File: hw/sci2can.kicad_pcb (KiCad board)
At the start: 2 copper layers, 31.1 x 32 mm, 34 parts, among them IC1 MC9S08DZ60xLC, J1 BDM, J2 Screw Terminal, Q1 4MHz, Q2 MGSF1N03L*, U1 uA7805, U2 PCA82C251

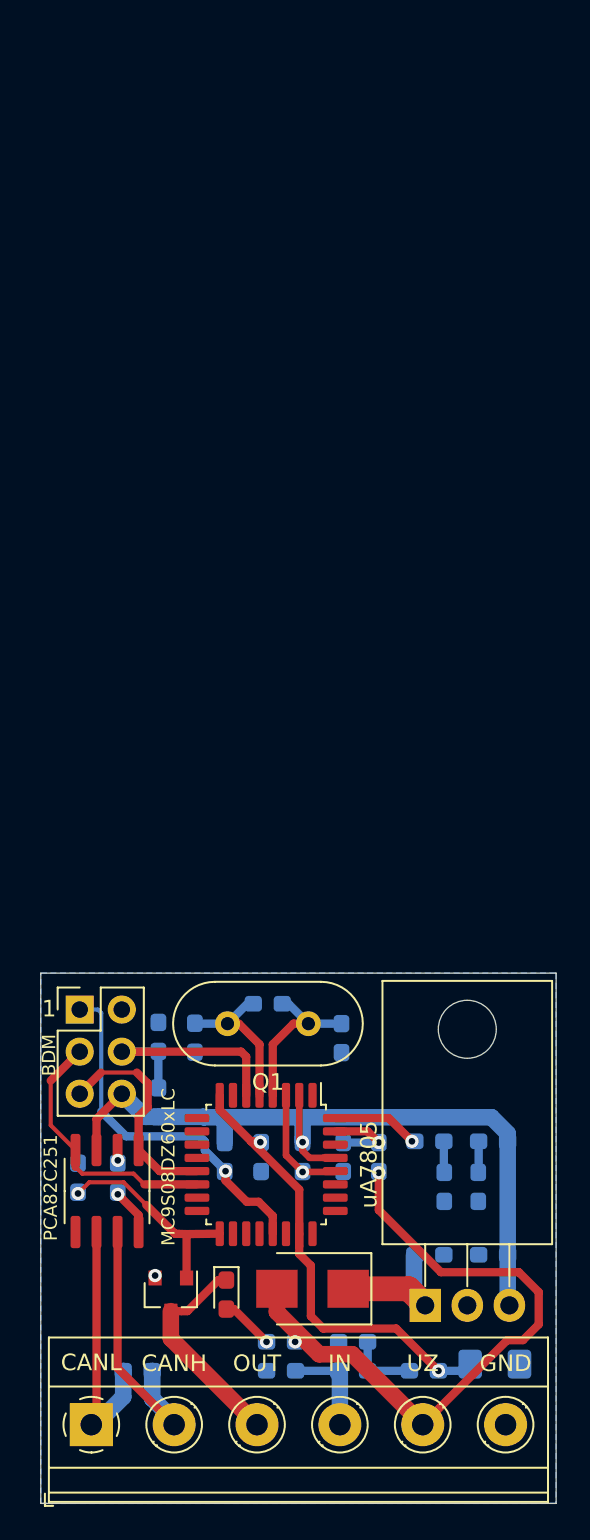
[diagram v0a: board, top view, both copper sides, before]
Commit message: hw 1v02
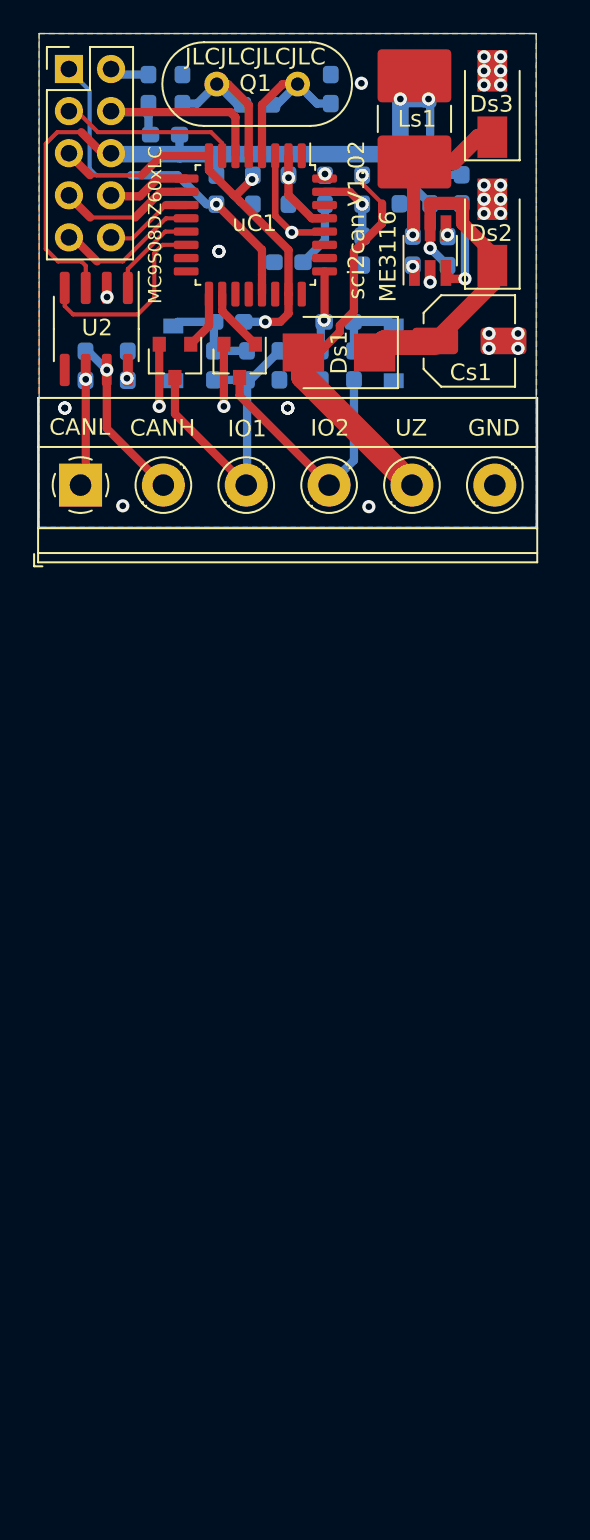
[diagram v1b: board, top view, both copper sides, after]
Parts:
- removed C1: 1uF, Capacitor_SMD:C_0603_1608Metric_Pad1.05x0.95mm_HandSolder
- removed C4: 22pF, Capacitor_SMD:C_0603_1608Metric_Pad1.05x0.95mm_HandSolder
- removed D1: LL4007, Diode_SMD:D_SMB
- removed D2: POWER*, Diode_SMD:D_0603_1608Metric_Pad1.05x0.95mm_HandSolder
- removed D3: STATUS, Diode_SMD:D_0603_1608Metric_Pad1.05x0.95mm_HandSolder
- removed D4: STOUT*, Diode_SMD:D_0603_1608Metric_Pad1.05x0.95mm_HandSolder
- removed IC1: MC9S08DZ60xLC, Package_QFP:LQFP-32_7x7mm_P0.8mm
- removed Q2: MGSF1N03L*, Package_TO_SOT_SMD:SOT-23
- removed R1: 680*, Resistor_SMD:R_0603_1608Metric_Pad1.05x0.95mm_HandSolder
- removed R13: 10k*, Resistor_SMD:R_0603_1608Metric_Pad1.05x0.95mm_HandSolder
- removed R14: 5k*, Resistor_SMD:R_0603_1608Metric_Pad1.05x0.95mm_HandSolder
- removed R8: 100, Resistor_SMD:R_0603_1608Metric_Pad1.05x0.95mm_HandSolder
- added Cq1: 22pF, Capacitor_SMD:C_0603_1608Metric_Pad1.05x0.95mm_HandSolder, B.Cu at (213.7, 79.0)
- added Cs1: 10uF 50V, Capacitor_SMD:C_Elec_5x5.8, F.Cu at (222.0, 94.2)
- added Cs2: 1uF, Capacitor_SMD:C_0603_1608Metric_Pad1.05x0.95mm_HandSolder, B.Cu at (218.6, 88.8)
- added Cs3: 220pF, Capacitor_SMD:C_0603_1608Metric_Pad1.05x0.95mm_HandSolder, B.Cu at (221.6, 85.1)
- added Cs6: 10uF, Capacitor_SMD:C_0603_1608Metric_Pad1.05x0.95mm_HandSolder, B.Cu at (217.8, 78.8)
- added Di1: BZT52C4V7, Diode_SMD:D_SOD-123, B.Cu at (217.4, 95.0)
- added Dl1: STATUS, Diode_SMD:D_0603_1608Metric_Pad1.05x0.95mm_HandSolder, B.Cu at (211.1, 89.5)
- added Ds1: LL4007, Diode_SMD:D_SMB, F.Cu at (214.2, 95.0)
- added Ds2: SMAJ33A 38.7V, Diode_SMD:D_SMA, F.Cu at (223.4, 87.7)
- added Ds3: SS34, Diode_SMD:D_SMA, F.Cu at (223.4, 80.0)
- added Ls1: 47uH, Inductor_SMD:L_2816_7142Metric_Pad3.20x4.45mm_HandSolder, F.Cu at (218.7, 80.8)
- added Rc1: 100, Resistor_SMD:R_0603_1608Metric_Pad1.05x0.95mm_HandSolder, B.Cu at (201.4, 95.8)
- added Ri7: 10k, Resistor_SMD:R_0603_1608Metric_Pad1.05x0.95mm_HandSolder, B.Cu at (215.1, 95.7)
- added Ri8: 1k, Resistor_SMD:R_0603_1608Metric_Pad1.05x0.95mm_HandSolder, B.Cu at (214.1, 93.1)
- added Ri9: ?*, Resistor_SMD:R_0603_1608Metric_Pad1.05x0.95mm_HandSolder, B.Cu at (213.1, 95.7)
- added Rs3: 1M, Resistor_SMD:R_0603_1608Metric_Pad1.05x0.95mm_HandSolder, B.Cu at (220.7, 88.8)
- added Rs4: 3k, Resistor_SMD:R_0603_1608Metric_Pad1.05x0.95mm_HandSolder, B.Cu at (217.8, 85.1)
- added Rs5: 10k, Resistor_SMD:R_0603_1608Metric_Pad1.05x0.95mm_HandSolder, B.Cu at (219.7, 85.1)
- added T1: TSM2308*, Package_TO_SOT_SMD:SOT-23, F.Cu at (208.2, 95.5)
- added T2: TSM2308*, Package_TO_SOT_SMD:SOT-23, F.Cu at (204.2, 95.5)
- added uC1: MC9S08DZ60xLC, Package_QFP:LQFP-32_7x7mm_P0.8mm, F.Cu at (209.1, 87.2)
- Cs4: renamed from C2; value 10nF -> 1uF
- Cs5: renamed from C3; value 1uF -> 10uF
- Di2: renamed from D5; value 4V7 -> BZT52C4V7; footprint Diode_SMD:D_1206_3216Metric_Pad1.42x1.75mm_HandSolder -> Diode_SMD:D_SOD-123
- J1: footprint Connector_PinHeader_2.54mm:PinHeader_2x03_P2.54mm_Vertical -> Connector_PinHeader_2.54mm:PinHeader_2x05_P2.54mm_Vertical
- Rb1: renamed from R10; value 10k* -> 10k
- Rc2: renamed from RT1; value 120 -> 100
- Ri4: renamed from R6; value Reserved* -> ?*
- Rl1: renamed from R12; value 680 -> 1k
- Rs1: renamed from R2; value 100k* -> 100k
- Rs2: renamed from R3; value 10k* -> 10k
- U1: value uA7805 -> ME3116; footprint Package_TO_SOT_THT:TO-220-3_Horizontal_TabDown -> Package_TO_SOT_SMD:SOT-23-6_Handsoldering
- moved Cs5 70.7 mm to (219.6, 78.8), turned to 90 degrees
- moved Ri3 64.4 mm to (207.5, 93.1)
- moved Di2 64.0 mm to (204.2, 95.0), turned to 270 degrees
- moved U1 63.7 mm to (219.7, 88.8), turned to 90 degrees
- moved Ri2 61.0 mm to (208.6, 95.7), turned to 270 degrees
- moved Rc2 60.7 mm to (198.8, 95.8), turned to 270 degrees
- moved Ri1 60.7 mm to (210.6, 95.7), turned to 270 degrees
- moved Ci2 59.5 mm to (206.6, 95.7), turned to 270 degrees
- moved Rr1 58.4 mm to (203.7, 81.8), turned to 0 degrees
- moved Rs1 58.4 mm to (215.6, 85.1), turned to 90 degrees
- moved Cs4 58.4 mm to (211.1, 85.1)
- moved Rb1 58.4 mm to (206.8, 85.1)
- moved Ri4 58.4 mm to (208.9, 85.1)
- moved Rl1 57.8 mm to (213.3, 85.1), turned to 270 degrees
- moved Cq2 57.3 mm to (204.7, 79.0), turned to 90 degrees
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- renumbered C7 to Ci2, C5 to Cq2, C6 to Cr1, R7 to Ri1, R4 to Ri2, R5 to Ri3, R9 to Rq1, R11 to Rr1
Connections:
- Ci2 pad 1: Net-(C7-Pad1) -> Net-(Ci2-Pad1)
- Ci2 pad 2: IN -> IO2
- Cs4 pad 1: +5V -> +3V3
- Cs5 pad 1: +5V -> +3V3
- Di2 pad 1: RxD1 -> Net-(Ci2-Pad1)
- J1 pad 3: RXCAN -> TxD1
- J1 pad 5: TXCAN -> RxD1
- J1 pad 6: +5V -> +3V3
- J2 pad 3: OUT -> IO2
- J2 pad 4: IN -> IO1
- Rb1 pad 1: +5V -> +3V3
- Ri1 pad 1: IN -> IO2
- Ri2 pad 1: Net-(C7-Pad1) -> Net-(Ci2-Pad1)
- Ri2 pad 2: IN -> IO2
- Ri3 pad 2: Net-(C7-Pad1) -> Net-(Ci2-Pad1)
- Rr1 pad 1: +5V -> RESET
- Rr1 pad 2: RESET -> +3V3
- U1 pad 3: +5V -> Net-(Cs3-Pad1)
- U2 pad 3: +5V -> +3V3
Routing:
- net +3V3: track 0.00 -> 53.0 mm, vias 0 -> 3
- net +5V: track 47.3 -> 0.00 mm, vias 1 -> 0
- net Net-(Cs1-Pad1): track 0.00 -> 20.7 mm, vias 0 -> 1
- net IO2: track 0.00 -> 19.3 mm
- net IO1: track 0.00 -> 15.7 mm
- net GND: track 8.17 -> 23.0 mm, vias 3 -> 31
- net UZ: track 39.3 -> 24.4 mm, vias 2 -> 1
- net OUT: track 13.1 -> 0.00 mm
- net FET: track 12.8 -> 0.00 mm, vias 1 -> 0
- net TxD1: track 0.00 -> 10.8 mm
- net Net-(Cs3-Pad1): track 0.00 -> 10.4 mm, vias 0 -> 1
- net Net-(Cs2-Pad2): track 0.00 -> 9.32 mm, vias 0 -> 1
- net SDA: track 0.00 -> 8.73 mm
- net CANL: track 15.8 -> 7.24 mm, vias 0 -> 1
- net PTE3: track 0.00 -> 8.25 mm
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- added copper zone on F.Cu, net GND
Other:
- board size 31.1 x 32 mm -> 30 x 29.8 mm
- board text added: "IO1"
- board text added: "IO2"
- board text added: "JLCJLCJLCJLC"
- board text added: "github/ butyi/ sci2can V1.02"
- board text added: "sci2can V1.02"
- board text removed: "1"
- board text removed: "IN"
- board text removed: "OUT"
- board text removed: "sci2can V1.01 2020.05.17 www.butyi.hu github.com/butyi/sci2can"
